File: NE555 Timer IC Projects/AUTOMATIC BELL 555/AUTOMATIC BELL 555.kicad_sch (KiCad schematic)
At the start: 12 parts, among them K1 SANYOU_SRD_Form_A, Q1 AO3400A, U1 LM555xM

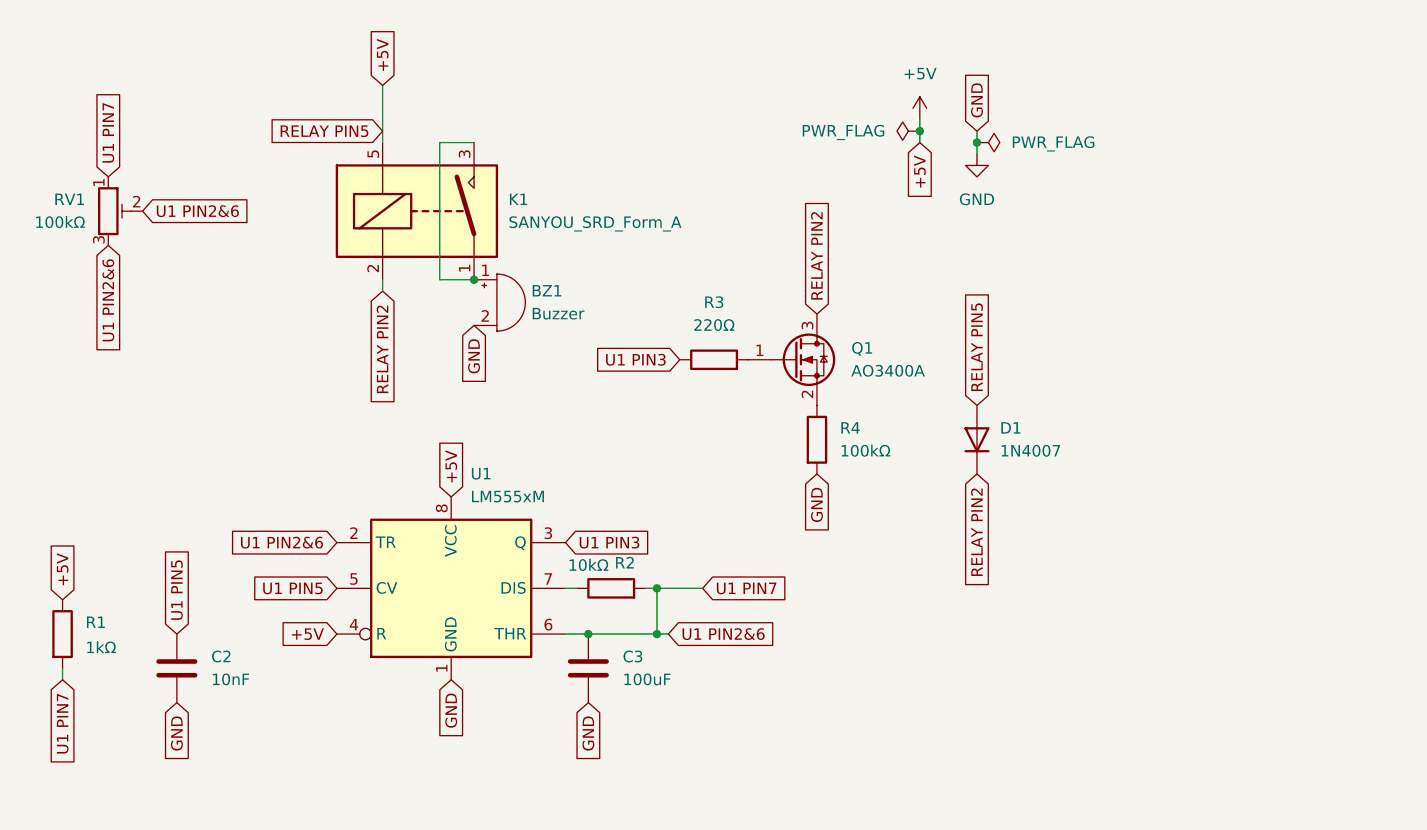
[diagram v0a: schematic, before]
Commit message: Initial Commit
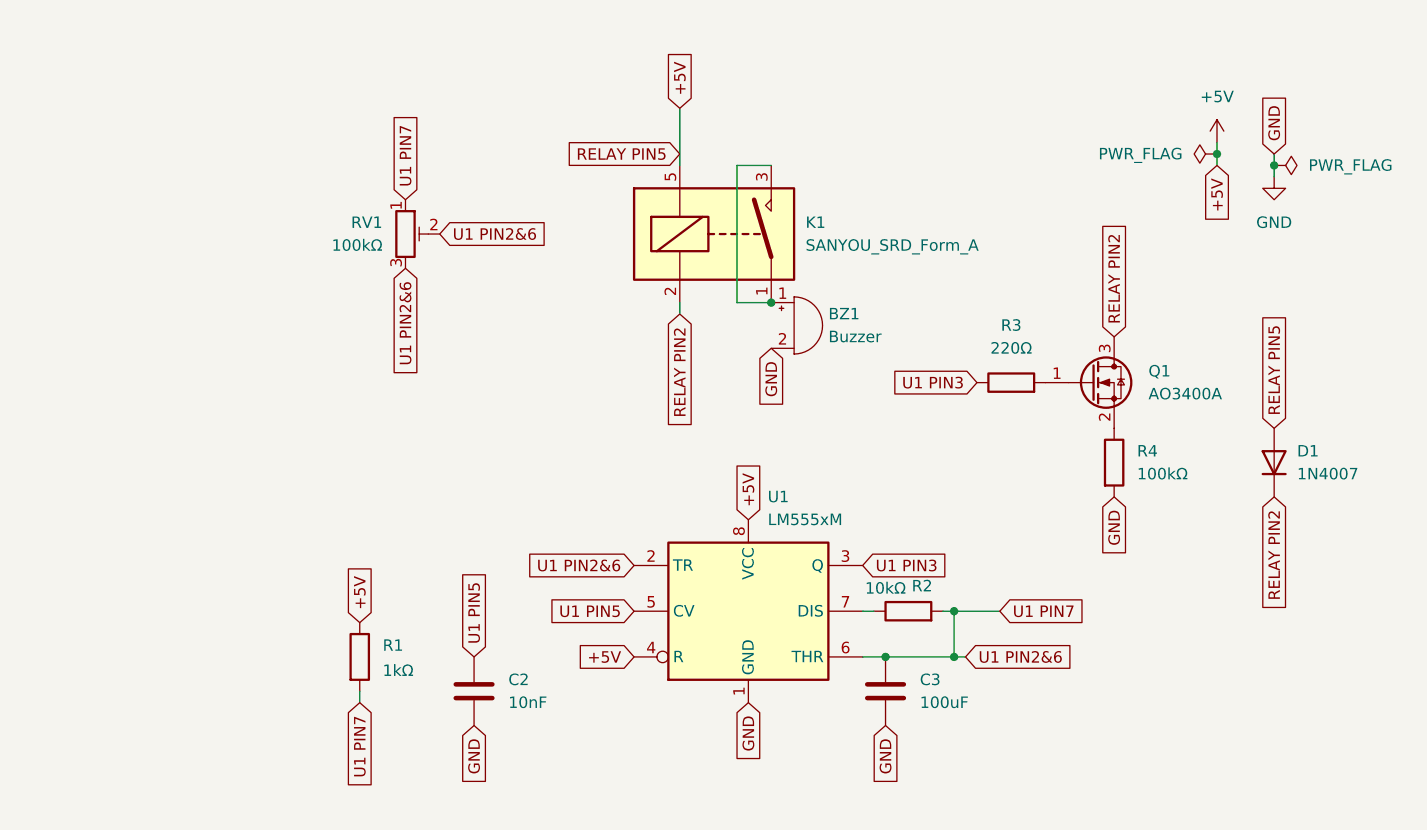
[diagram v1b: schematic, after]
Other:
- moved on the sheet: BZ1, C2, C3, D1, K1, Q1, R1, R2, R3, R4, RV1, U1
